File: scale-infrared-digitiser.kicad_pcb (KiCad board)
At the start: 2 copper layers, 175 x 47.5 mm, 389 parts, among them IC0 LM324PT, IC1 LM324PT, IC2 LM324PT, IC3 LM324PT, IC4 74HC4067PW,118, IC5 74HC4067PW,118, J0 Conn_02x04_TRNS, J1 Conn_02x04_RECV, Q1 T2N7002AK, Q10 T2N7002AK, Q11 T2N7002AK, Q12 T2N7002AK, Q13 T2N7002AK, Q14 T2N7002AK, Q15 T2N7002AK, Q16 T2N7002AK, Q2 T2N7002AK, Q3 T2N7002AK, Q4 T2N7002AK, Q5 T2N7002AK, Q6 T2N7002AK, Q7 T2N7002AK, Q8 T2N7002AK, Q9 T2N7002AK

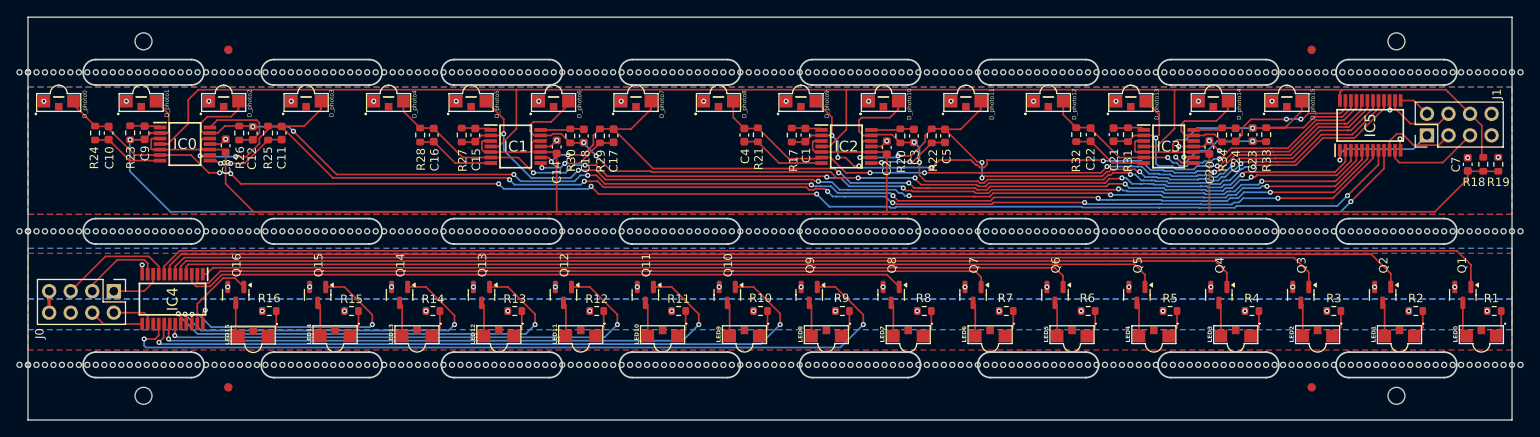
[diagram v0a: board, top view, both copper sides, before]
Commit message: revised DFM submitted to JLCPCB
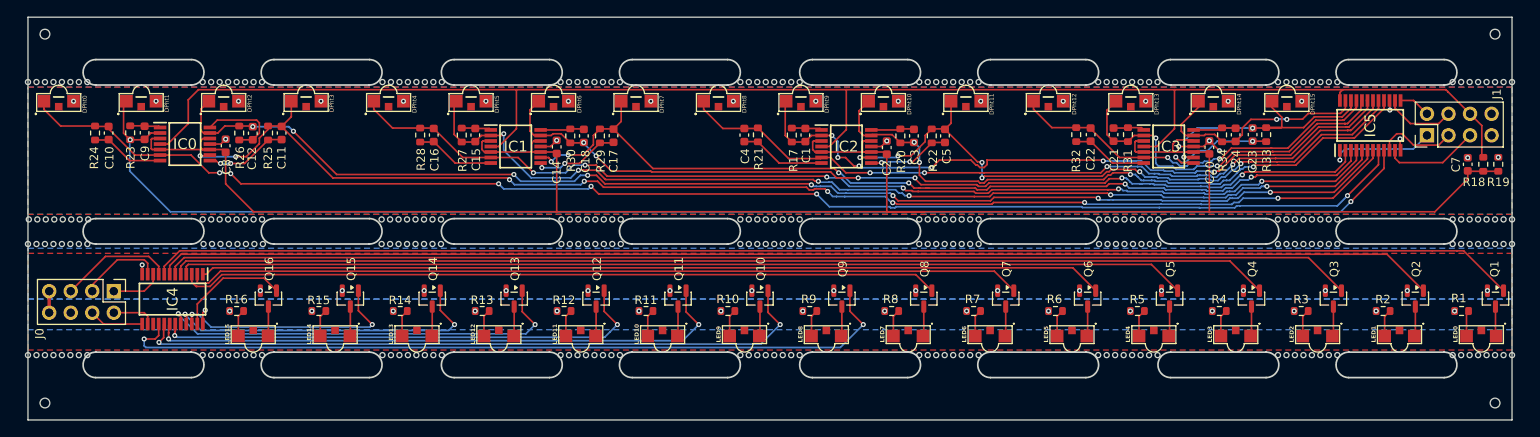
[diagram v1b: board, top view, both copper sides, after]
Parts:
- removed ? (x3): , 
- removed the REF** at (137.0, 91.2)
- removed the REF** at (173.0, 110.0)
- removed the REF** at (147.0, 110.0)
- removed the REF** at (117.0, 91.2)
- removed the REF** at (217.4, 88.6)
- removed the REF** at (103.0, 91.2)
- removed the REF** at (97.0, 125.8)
- removed the REF** at (185.0, 91.2)
- removed the REF** at (75.0, 91.2)
- removed the REF** at (131.0, 125.8)
- removed the REF** at (131.0, 110.0)
- removed the REF** at (85.0, 91.2)
- removed the REF** at (233.0, 110.0)
- removed the REF** at (123.0, 125.8)
- removed the REF** at (237.0, 91.2)
- removed the REF** at (85.0, 110.0)
- removed the REF** at (205.0, 91.2)
- removed the REF** at (201.0, 110.0)
- removed the REF** at (97.0, 110.0)
- removed the REF** at (149.0, 91.2)
- removed the REF** at (91.0, 110.0)
- removed the REF** at (185.0, 110.0)
- removed the REF** at (225.0, 110.0)
- removed the REF** at (205.0, 110.0)
- removed the REF** at (181.0, 125.8)
- removed the REF** at (121.0, 125.8)
- removed the REF** at (79.0, 125.8)
- removed the REF** at (197.0, 91.2)
- removed the REF** at (83.0, 110.0)
- removed the REF** at (183.0, 125.8)
- removed the REF** at (77.0, 110.0)
- removed the REF** at (175.0, 110.0)
- removed the REF** at (205.0, 125.8)
- removed the REF** at (71.0, 110.0)
- removed the REF** at (93.0, 91.2)
- removed the REF** at (143.0, 91.2)
- removed the REF** at (185.0, 125.8)
- removed the REF** at (127.0, 91.2)
- removed the REF** at (215.0, 110.0)
- removed the REF** at (215.0, 125.8)
- removed the REF** at (197.0, 110.0)
- removed the REF** at (89.0, 125.8)
- removed the REF** at (209.0, 125.8)
- removed the REF** at (191.0, 110.0)
- removed the REF** at (227.4, 129.4)
- removed the REF** at (219.0, 91.2)
- removed the REF** at (89.0, 91.2)
- removed the REF** at (211.0, 91.2)
- removed the REF** at (101.0, 110.0)
- removed the REF** at (183.0, 91.2)
- removed the REF** at (115.0, 125.8)
- removed the REF** at (235.0, 110.0)
- removed the REF** at (235.0, 125.8)
- removed the REF** at (119.0, 91.2)
- removed the REF** at (195.0, 125.8)
- removed the REF** at (159.0, 91.2)
- removed the REF** at (161.0, 110.0)
- removed the REF** at (123.0, 110.0)
- removed the REF** at (79.0, 91.2)
- removed the REF** at (107.0, 125.8)
- removed the REF** at (147.0, 125.8)
- removed the REF** at (227.4, 87.6)
- removed the REF** at (241.0, 110.0)
- removed the REF** at (171.0, 110.0)
- removed the REF** at (167.0, 91.2)
- removed the REF** at (223.0, 110.0)
- removed the REF** at (67.0, 125.8)
- removed the REF** at (75.0, 110.0)
- removed the REF** at (119.0, 125.8)
- removed the REF** at (211.0, 110.0)
- removed the REF** at (237.0, 110.0)
- removed the REF** at (157.0, 91.2)
- removed the REF** at (153.0, 91.2)
- removed the REF** at (197.0, 125.8)
- removed the REF** at (113.0, 125.8)
- removed the REF** at (71.0, 91.2)
- removed the REF** at (225.0, 125.8)
- removed the REF** at (227.0, 125.8)
- removed the REF** at (165.0, 110.0)
- removed the REF** at (101.0, 91.2)
- removed the REF** at (113.0, 110.0)
- removed the REF** at (91.0, 91.2)
- removed the REF** at (67.0, 91.2)
- removed the REF** at (115.0, 91.2)
- removed the REF** at (175.0, 125.8)
- removed the REF** at (105.0, 91.2)
- removed the REF** at (221.0, 125.8)
- removed the REF** at (233.0, 125.8)
- removed the REF** at (165.0, 125.8)
- removed the REF** at (111.0, 110.0)
- removed the REF** at (167.0, 125.8)
- removed the REF** at (133.0, 125.8)
- removed the REF** at (105.0, 125.8)
- removed the REF** at (169.0, 125.8)
- removed the REF** at (151.0, 91.2)
- removed the REF** at (135.0, 91.2)
- removed the REF** at (83.0, 125.8)
- removed the REF** at (151.0, 110.0)
- removed the REF** at (173.0, 125.8)
- removed the REF** at (93.0, 110.0)
- removed the REF** at (227.0, 91.2)
- removed the REF** at (71.0, 125.8)
- removed the REF** at (171.0, 91.2)
- removed the REF** at (89.6, 88.6)
- removed the REF** at (223.0, 91.2)
- removed the REF** at (89.0, 110.0)
- removed the REF** at (129.0, 125.8)
- removed the REF** at (99.0, 125.8)
- removed the REF** at (169.0, 110.0)
- removed the REF** at (111.0, 91.2)
- removed the REF** at (97.0, 91.2)
- removed the REF** at (217.0, 125.8)
- removed the REF** at (95.0, 110.0)
- removed the REF** at (229.0, 110.0)
- removed the REF** at (81.0, 110.0)
- removed the REF** at (81.0, 91.2)
- removed the REF** at (191.0, 91.2)
- removed the REF** at (109.0, 91.2)
- removed the REF** at (95.0, 91.2)
- removed the REF** at (145.0, 110.0)
- removed the REF** at (155.0, 91.2)
- removed the REF** at (111.0, 125.8)
- removed the REF** at (183.0, 110.0)
- removed the REF** at (79.6, 87.6)
- removed the REF** at (209.0, 110.0)
- removed the REF** at (201.0, 125.8)
- removed the REF** at (189.0, 110.0)
- removed the REF** at (115.0, 110.0)
- removed the REF** at (227.0, 110.0)
- removed the REF** at (229.0, 91.2)
- removed the REF** at (145.0, 91.2)
- removed the REF** at (171.0, 125.8)
- removed the REF** at (151.0, 125.8)
- removed the REF** at (211.0, 125.8)
- removed the REF** at (239.0, 91.2)
- removed the REF** at (241.0, 125.8)
- removed the REF** at (137.0, 125.8)
- removed the REF** at (155.0, 110.0)
- removed the REF** at (65.0, 91.2)
- removed the REF** at (157.0, 125.8)
- removed the REF** at (135.0, 125.8)
- removed the REF** at (207.0, 125.8)
- removed the REF** at (73.0, 110.0)
- removed the REF** at (159.0, 110.0)
- removed the REF** at (181.0, 91.2)
- removed the REF** at (135.0, 110.0)
- removed the REF** at (179.0, 125.8)
- removed the REF** at (173.0, 91.2)
- removed the REF** at (239.0, 110.0)
- removed the REF** at (121.0, 91.2)
- removed the REF** at (177.0, 91.2)
- removed the REF** at (233.0, 91.2)
- removed the REF** at (125.0, 125.8)
- removed the REF** at (161.0, 125.8)
- removed the REF** at (89.6, 128.4)
- removed the REF** at (189.0, 125.8)
- removed the REF** at (217.4, 128.4)
- removed the REF** at (137.0, 110.0)
- removed the REF** at (147.0, 91.2)
- removed the REF** at (163.0, 91.2)
- removed the REF** at (109.0, 110.0)
- removed the REF** at (163.0, 125.8)
- removed the REF** at (79.0, 110.0)
- removed the REF** at (101.0, 125.8)
- removed the REF** at (83.0, 91.2)
- removed the REF** at (181.0, 110.0)
- removed the REF** at (75.0, 125.8)
- removed the REF** at (221.0, 110.0)
- removed the REF** at (239.0, 125.8)
- removed the REF** at (179.0, 91.2)
- removed the REF** at (133.0, 110.0)
- removed the REF** at (65.0, 110.0)
- removed the REF** at (207.0, 110.0)
- removed the REF** at (189.0, 91.2)
- removed the REF** at (209.0, 91.2)
- removed the REF** at (237.0, 125.8)
- removed the REF** at (131.0, 91.2)
- removed the REF** at (117.0, 110.0)
- removed the REF** at (177.0, 110.0)
- removed the REF** at (175.0, 91.2)
- removed the REF** at (77.0, 125.8)
- removed the REF** at (123.0, 91.2)
- removed the REF** at (215.0, 91.2)
- removed the REF** at (103.0, 110.0)
- removed the REF** at (73.0, 91.2)
- removed the REF** at (95.0, 125.8)
- removed the REF** at (203.0, 125.8)
- removed the REF** at (77.0, 91.2)
- removed the REF** at (67.0, 110.0)
- removed the REF** at (155.0, 125.8)
- removed the REF** at (187.0, 91.2)
- removed the REF** at (163.0, 110.0)
- removed the REF** at (143.0, 110.0)
- removed the REF** at (87.0, 91.2)
- removed the REF** at (219.0, 110.0)
- removed the REF** at (191.0, 125.8)
- removed the REF** at (221.0, 91.2)
- removed the REF** at (133.0, 91.2)
- removed the REF** at (103.0, 125.8)
- removed the REF** at (65.0, 125.8)
- removed the REF** at (199.0, 110.0)
- removed the REF** at (141.0, 91.2)
- removed the REF** at (139.0, 110.0)
- removed the REF** at (153.0, 125.8)
- removed the REF** at (125.0, 110.0)
- removed the REF** at (69.0, 110.0)
- removed the REF** at (223.0, 125.8)
- removed the REF** at (145.0, 125.8)
- removed the REF** at (125.0, 91.2)
- removed the REF** at (195.0, 91.2)
- removed the REF** at (213.0, 91.2)
- removed the REF** at (99.0, 110.0)
- removed the REF** at (203.0, 110.0)
- removed the REF** at (69.0, 91.2)
- removed the REF** at (79.6, 129.4)
- removed the REF** at (127.0, 110.0)
- removed the REF** at (217.0, 110.0)
- removed the REF** at (187.0, 125.8)
- removed the REF** at (203.0, 91.2)
- removed the REF** at (235.0, 91.2)
- removed the REF** at (87.0, 125.8)
- removed the REF** at (129.0, 110.0)
- removed the REF** at (207.0, 91.2)
- removed the REF** at (217.0, 91.2)
- removed the REF** at (91.0, 125.8)
- removed the REF** at (193.0, 91.2)
- removed the REF** at (85.0, 125.8)
- removed the REF** at (117.0, 125.8)
- removed the REF** at (179.0, 110.0)
- removed the REF** at (231.0, 91.2)
- removed the REF** at (199.0, 125.8)
- removed the REF** at (139.0, 125.8)
- removed the REF** at (241.0, 91.2)
- removed the REF** at (231.0, 110.0)
- removed the REF** at (69.0, 125.8)
- removed the REF** at (159.0, 125.8)
- removed the REF** at (199.0, 91.2)
- removed the REF** at (107.0, 91.2)
- removed the REF** at (187.0, 110.0)
- removed the REF** at (149.0, 125.8)
- removed the REF** at (99.0, 91.2)
- removed the REF** at (143.0, 125.8)
- removed the REF** at (73.0, 125.8)
- removed the REF** at (141.0, 125.8)
- removed the REF** at (201.0, 91.2)
- removed the REF** at (193.0, 125.8)
- removed the REF** at (177.0, 125.8)
- removed the REF** at (195.0, 110.0)
- removed the REF** at (149.0, 110.0)
- removed the REF** at (157.0, 110.0)
- removed the REF** at (167.0, 110.0)
- removed the REF** at (129.0, 91.2)
- removed the REF** at (107.0, 110.0)
- removed the REF** at (109.0, 125.8)
- removed the REF** at (113.0, 91.2)
- removed the REF** at (141.0, 110.0)
- removed the REF** at (225.0, 91.2)
- removed the REF** at (121.0, 110.0)
- removed the REF** at (169.0, 91.2)
- removed the REF** at (213.0, 110.0)
- removed the REF** at (213.0, 125.8)
- removed the REF** at (93.0, 125.8)
- removed the REF** at (153.0, 110.0)
- removed the REF** at (139.0, 91.2)
- removed the REF** at (87.0, 110.0)
- removed the REF** at (127.0, 125.8)
- removed the REF** at (229.0, 125.8)
- removed the REF** at (219.0, 125.8)
- removed the REF** at (193.0, 110.0)
- removed the REF** at (81.0, 125.8)
- removed the REF** at (105.0, 110.0)
- removed the REF** at (231.0, 125.8)
- removed the REF** at (161.0, 91.2)
- removed the REF** at (165.0, 91.2)
- removed the REF** at (119.0, 110.0)
- added REF**: mouse_bites, manufacturing:mouse_bites, F.Cu at (234.0, 92.4)
- added REF**: mouse_bites, manufacturing:mouse_bites, F.Cu at (128.8, 92.4)
- added REF**: mouse_bites, manufacturing:mouse_bites, F.Cu at (92.6, 92.4)
- added REF**: mouse_bites, manufacturing:mouse_bites, F.Cu at (213.4, 92.4)
- added REF**: mouse_bites, manufacturing:mouse_bites, F.Cu at (133.8, 124.6)
- added REF**: mouse_bites, manufacturing:mouse_bites, F.Cu at (177.1, 108.6)
- added REF**: mouse_bites, manufacturing:mouse_bites, F.Cu at (128.8, 124.6)
- added REF**: mouse_bites, manufacturing:mouse_bites, F.Cu at (134.9, 108.6)
- added REF**: mouse_bites, manufacturing:mouse_bites, F.Cu at (156.0, 92.4)
- added REF**: mouse_bites, manufacturing:mouse_bites, F.Cu at (113.7, 108.6)
- added REF**: mouse_bites, manufacturing:mouse_bites, F.Cu at (199.2, 124.6)
- added REF**: mouse_bites, manufacturing:mouse_bites, F.Cu at (66.0, 111.5)
- added REF**: mouse_bites, manufacturing:mouse_bites, F.Cu at (112.7, 108.6)
- added REF**: mouse_bites, manufacturing:mouse_bites, F.Cu at (171.1, 124.6)
- added REF**: mouse_bites, manufacturing:mouse_bites, F.Cu at (239.0, 111.5)
- added REF**: mouse_bites, manufacturing:mouse_bites, F.Cu at (237.0, 124.6)
- added REF**: mouse_bites, manufacturing:mouse_bites, F.Cu at (218.4, 111.5)
- added REF**: mouse_bites, manufacturing:mouse_bites, F.Cu at (134.9, 111.5)
- added REF**: ToolingHole_1.152mm, MountingHole:ToolingHole_1.152mm, F.Cu at (68.0, 86.8)
- added REF**: mouse_bites, manufacturing:mouse_bites, F.Cu at (91.7, 111.5)
- added REF**: mouse_bites, manufacturing:mouse_bites, F.Cu at (219.4, 124.6)
- added REF**: mouse_bites, manufacturing:mouse_bites, F.Cu at (112.8, 124.6)
- added REF**: mouse_bites, manufacturing:mouse_bites, F.Cu at (69.0, 111.5)
- added REF**: mouse_bites, manufacturing:mouse_bites, F.Cu at (234.0, 108.6)
- added REF**: mouse_bites, manufacturing:mouse_bites, F.Cu at (112.7, 111.5)
- added REF**: mouse_bites, manufacturing:mouse_bites, F.Cu at (176.1, 92.4)
- added REF**: mouse_bites, manufacturing:mouse_bites, F.Cu at (69.0, 124.6)
- added REF**: mouse_bites, manufacturing:mouse_bites, F.Cu at (237.0, 111.5)
- added REF**: mouse_bites, manufacturing:mouse_bites, F.Cu at (213.4, 111.5)
- added REF**: mouse_bites, manufacturing:mouse_bites, F.Cu at (113.8, 124.6)
- added REF**: mouse_bites, manufacturing:mouse_bites, F.Cu at (150.0, 92.4)
- added REF**: mouse_bites, manufacturing:mouse_bites, F.Cu at (194.2, 124.6)
- added REF**: mouse_bites, manufacturing:mouse_bites, F.Cu at (171.1, 111.5)
- added REF**: mouse_bites, manufacturing:mouse_bites, F.Cu at (197.3, 108.6)
- added REF**: mouse_bites, manufacturing:mouse_bites, F.Cu at (197.3, 111.5)
- added REF**: mouse_bites, manufacturing:mouse_bites, F.Cu at (216.4, 92.4)
- added REF**: mouse_bites, manufacturing:mouse_bites, F.Cu at (107.7, 111.5)
- added REF**: mouse_bites, manufacturing:mouse_bites, F.Cu at (240.0, 124.6)
- added REF**: mouse_bites, manufacturing:mouse_bites, F.Cu at (234.0, 111.5)
- added REF**: mouse_bites, manufacturing:mouse_bites, F.Cu at (174.1, 92.4)
- added REF**: mouse_bites, manufacturing:mouse_bites, F.Cu at (69.1, 108.6)
- added REF**: mouse_bites, manufacturing:mouse_bites, F.Cu at (155.0, 92.4)
- added REF**: mouse_bites, manufacturing:mouse_bites, F.Cu at (72.0, 124.6)
- added REF**: mouse_bites, manufacturing:mouse_bites, F.Cu at (71.0, 92.4)
- added REF**: mouse_bites, manufacturing:mouse_bites, F.Cu at (237.0, 108.6)
- added REF**: mouse_bites, manufacturing:mouse_bites, F.Cu at (213.4, 124.6)
- added REF**: mouse_bites, manufacturing:mouse_bites, F.Cu at (69.0, 92.4)
- added REF**: mouse_bites, manufacturing:mouse_bites, F.Cu at (239.0, 108.6)
- added REF**: mouse_bites, manufacturing:mouse_bites, F.Cu at (110.7, 111.5)
- added REF**: mouse_bites, manufacturing:mouse_bites, F.Cu at (107.8, 92.4)
- added REF**: mouse_bites, manufacturing:mouse_bites, F.Cu at (89.7, 111.5)
- added REF**: mouse_bites, manufacturing:mouse_bites, F.Cu at (153.0, 124.6)
- added REF**: mouse_bites, manufacturing:mouse_bites, F.Cu at (156.0, 108.6)
- added REF**: mouse_bites, manufacturing:mouse_bites, F.Cu at (194.2, 92.4)
- added REF**: mouse_bites, manufacturing:mouse_bites, F.Cu at (92.6, 124.6)
- added REF**: mouse_bites, manufacturing:mouse_bites, F.Cu at (177.1, 111.5)
- added REF**: mouse_bites, manufacturing:mouse_bites, F.Cu at (219.4, 111.5)
- added REF**: mouse_bites, manufacturing:mouse_bites, F.Cu at (131.9, 111.5)
- added REF**: mouse_bites, manufacturing:mouse_bites, F.Cu at (133.9, 111.5)
- added REF**: mouse_bites, manufacturing:mouse_bites, F.Cu at (72.0, 111.5)
- added REF**: mouse_bites, manufacturing:mouse_bites, F.Cu at (171.1, 92.4)
- added REF**: mouse_bites, manufacturing:mouse_bites, F.Cu at (153.0, 92.4)
- added REF**: mouse_bites, manufacturing:mouse_bites, F.Cu at (134.8, 124.6)
- added REF**: mouse_bites, manufacturing:mouse_bites, F.Cu at (71.0, 111.5)
- added REF**: mouse_bites, manufacturing:mouse_bites, F.Cu at (150.0, 124.6)
- added REF**: mouse_bites, manufacturing:mouse_bites, F.Cu at (239.0, 124.6)
- added REF**: mouse_bites, manufacturing:mouse_bites, F.Cu at (91.6, 124.6)
- added REF**: mouse_bites, manufacturing:mouse_bites, F.Cu at (174.1, 111.5)
- added REF**: mouse_bites, manufacturing:mouse_bites, F.Cu at (72.1, 108.6)
- added REF**: mouse_bites, manufacturing:mouse_bites, F.Cu at (195.3, 108.6)
- added REF**: mouse_bites, manufacturing:mouse_bites, F.Cu at (86.6, 108.6)
- added REF**: mouse_bites, manufacturing:mouse_bites, F.Cu at (150.0, 111.5)
- added REF**: mouse_bites, manufacturing:mouse_bites, F.Cu at (155.0, 111.5)
- added REF**: mouse_bites, manufacturing:mouse_bites, F.Cu at (216.4, 124.6)
- added REF**: mouse_bites, manufacturing:mouse_bites, F.Cu at (89.6, 124.6)
- added REF**: mouse_bites, manufacturing:mouse_bites, F.Cu at (216.4, 108.6)
- added REF**: mouse_bites, manufacturing:mouse_bites, F.Cu at (240.0, 92.4)
- added REF**: mouse_bites, manufacturing:mouse_bites, F.Cu at (86.7, 111.5)
- added REF**: mouse_bites, manufacturing:mouse_bites, F.Cu at (155.0, 108.6)
- added REF**: mouse_bites, manufacturing:mouse_bites, F.Cu at (219.4, 108.6)
- added REF**: mouse_bites, manufacturing:mouse_bites, F.Cu at (174.1, 108.6)
- added REF**: mouse_bites, manufacturing:mouse_bites, F.Cu at (240.0, 111.5)
- added REF**: mouse_bites, manufacturing:mouse_bites, F.Cu at (192.3, 111.5)
- added REF**: mouse_bites, manufacturing:mouse_bites, F.Cu at (177.1, 92.4)
- added REF**: mouse_bites, manufacturing:mouse_bites, F.Cu at (113.8, 92.4)
- added REF**: mouse_bites, manufacturing:mouse_bites, F.Cu at (174.1, 124.6)
- added REF**: mouse_bites, manufacturing:mouse_bites, F.Cu at (150.0, 108.6)
- added REF**: mouse_bites, manufacturing:mouse_bites, F.Cu at (91.6, 92.4)
- added REF**: mouse_bites, manufacturing:mouse_bites, F.Cu at (192.3, 108.6)
- added REF**: mouse_bites, manufacturing:mouse_bites, F.Cu at (131.8, 124.6)
- added REF**: mouse_bites, manufacturing:mouse_bites, F.Cu at (134.8, 92.4)
- added REF**: mouse_bites, manufacturing:mouse_bites, F.Cu at (89.6, 108.6)
- added REF**: mouse_bites, manufacturing:mouse_bites, F.Cu at (198.3, 111.5)
- added REF**: mouse_bites, manufacturing:mouse_bites, F.Cu at (153.0, 108.6)
- added REF**: mouse_bites, manufacturing:mouse_bites, F.Cu at (110.7, 108.6)
- added REF**: mouse_bites, manufacturing:mouse_bites, F.Cu at (176.1, 108.6)
- added REF**: mouse_bites, manufacturing:mouse_bites, F.Cu at (110.8, 92.4)
- added REF**: mouse_bites, manufacturing:mouse_bites, F.Cu at (156.0, 124.6)
- added REF**: mouse_bites, manufacturing:mouse_bites, F.Cu at (193.2, 124.6)
- added REF**: mouse_bites, manufacturing:mouse_bites, F.Cu at (128.9, 108.6)
- added REF**: mouse_bites, manufacturing:mouse_bites, F.Cu at (133.8, 92.4)
- added REF**: mouse_bites, manufacturing:mouse_bites, F.Cu at (71.1, 108.6)
- added REF**: mouse_bites, manufacturing:mouse_bites, F.Cu at (107.7, 108.6)
- added REF**: mouse_bites, manufacturing:mouse_bites, F.Cu at (89.6, 92.4)
- added REF**: mouse_bites, manufacturing:mouse_bites, F.Cu at (218.4, 124.6)
- added REF**: mouse_bites, manufacturing:mouse_bites, F.Cu at (66.1, 108.6)
- added REF**: mouse_bites, manufacturing:mouse_bites, F.Cu at (131.9, 108.6)
- added REF**: mouse_bites, manufacturing:mouse_bites, F.Cu at (71.0, 124.6)
- added REF**: mouse_bites, manufacturing:mouse_bites, F.Cu at (176.1, 111.5)
- added REF**: mouse_bites, manufacturing:mouse_bites, F.Cu at (237.0, 92.4)
- added REF**: mouse_bites, manufacturing:mouse_bites, F.Cu at (66.0, 124.6)
- added REF**: mouse_bites, manufacturing:mouse_bites, F.Cu at (107.8, 124.6)
- added REF**: mouse_bites, manufacturing:mouse_bites, F.Cu at (156.0, 111.5)
- added REF**: mouse_bites, manufacturing:mouse_bites, F.Cu at (112.8, 92.4)
- added REF**: ToolingHole_1.152mm, MountingHole:ToolingHole_1.152mm, F.Cu at (239.0, 86.8)
- added REF**: mouse_bites, manufacturing:mouse_bites, F.Cu at (171.1, 108.6)
- added REF**: mouse_bites, manufacturing:mouse_bites, F.Cu at (196.2, 92.4)
- added REF**: mouse_bites, manufacturing:mouse_bites, F.Cu at (213.4, 108.6)
- added REF**: mouse_bites, manufacturing:mouse_bites, F.Cu at (216.4, 111.5)
- added REF**: mouse_bites, manufacturing:mouse_bites, F.Cu at (176.1, 124.6)
- added REF**: mouse_bites, manufacturing:mouse_bites, F.Cu at (133.9, 108.6)
- added REF**: mouse_bites, manufacturing:mouse_bites, F.Cu at (66.0, 92.4)
- added REF**: mouse_bites, manufacturing:mouse_bites, F.Cu at (198.3, 108.6)
- added REF**: mouse_bites, manufacturing:mouse_bites, F.Cu at (240.0, 108.6)
- added REF**: mouse_bites, manufacturing:mouse_bites, F.Cu at (199.2, 92.4)
- added REF**: mouse_bites, manufacturing:mouse_bites, F.Cu at (113.7, 111.5)
- added REF**: mouse_bites, manufacturing:mouse_bites, F.Cu at (193.2, 92.4)
- added REF**: mouse_bites, manufacturing:mouse_bites, F.Cu at (155.0, 124.6)
- added REF**: mouse_bites, manufacturing:mouse_bites, F.Cu at (86.6, 92.4)
- added REF**: mouse_bites, manufacturing:mouse_bites, F.Cu at (234.0, 124.6)
- added REF**: mouse_bites, manufacturing:mouse_bites, F.Cu at (218.4, 92.4)
- added REF**: mouse_bites, manufacturing:mouse_bites, F.Cu at (239.0, 92.4)
- added REF**: mouse_bites, manufacturing:mouse_bites, F.Cu at (86.6, 124.6)
- added REF**: mouse_bites, manufacturing:mouse_bites, F.Cu at (131.8, 92.4)
- added REF**: mouse_bites, manufacturing:mouse_bites, F.Cu at (177.1, 124.6)
- added REF**: mouse_bites, manufacturing:mouse_bites, F.Cu at (195.3, 111.5)
- added REF**: ToolingHole_1.152mm, MountingHole:ToolingHole_1.152mm, F.Cu at (239.0, 130.2)
- added REF**: mouse_bites, manufacturing:mouse_bites, F.Cu at (153.0, 111.5)
- added REF**: mouse_bites, manufacturing:mouse_bites, F.Cu at (110.8, 124.6)
- added REF**: mouse_bites, manufacturing:mouse_bites, F.Cu at (72.0, 92.4)
- added REF**: mouse_bites, manufacturing:mouse_bites, F.Cu at (92.6, 108.6)
- added REF**: mouse_bites, manufacturing:mouse_bites, F.Cu at (128.9, 111.5)
- added REF**: mouse_bites, manufacturing:mouse_bites, F.Cu at (218.4, 108.6)
- added REF**: ToolingHole_1.152mm, MountingHole:ToolingHole_1.152mm, F.Cu at (68.0, 130.2)
- added REF**: mouse_bites, manufacturing:mouse_bites, F.Cu at (92.7, 111.5)
- added REF**: mouse_bites, manufacturing:mouse_bites, F.Cu at (219.4, 92.4)
- added REF**: mouse_bites, manufacturing:mouse_bites, F.Cu at (196.2, 124.6)
- added REF**: mouse_bites, manufacturing:mouse_bites, F.Cu at (91.6, 108.6)
- moved Q1 3.87 mm to (239.1, 117.9)
- moved Q10 3.87 mm to (152.3, 117.9)
- moved Q3 3.87 mm to (219.9, 117.9)
- moved Q13 3.87 mm to (123.3, 117.9)
- moved Q14 3.87 mm to (113.7, 117.9)
- moved Q11 3.87 mm to (142.7, 117.9)
- moved Q12 3.87 mm to (133.0, 117.9)
- moved Q15 3.87 mm to (104.0, 117.9)
- moved Q16 3.87 mm to (94.3, 117.9)
- moved Q2 3.87 mm to (229.6, 117.9)
- moved Q4 3.87 mm to (210.3, 117.9)
- moved Q5 3.87 mm to (200.6, 117.9)
- moved Q6 3.87 mm to (191.0, 117.9)
- moved Q7 3.87 mm to (181.3, 117.9)
- moved Q8 3.87 mm to (171.6, 117.9)
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- renumbered D_photo0 to DPht0, D_photo1 to DPht1, D_photo10 to DPht10, D_photo11 to DPht11, D_photo12 to DPht12, D_photo13 to DPht13, D_photo14 to DPht14, D_photo15 to DPht15, D_photo2 to DPht2, D_photo3 to DPht3, D_photo4 to DPht4, D_photo5 to DPht5, D_photo6 to DPht6, D_photo7 to DPht7, D_photo8 to DPht8, D_photo9 to DPht9
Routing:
- net /LED_CTL_7: track 85.7 -> 89.8 mm
- net /LED_CTL_15: track 9.55 -> 13.6 mm
- net /PHT_DAT_1: track 163.6 -> 167.5 mm
- net /PHT_DAT_15: track 79.5 -> 76.1 mm
- net /PHT_DAT_5: track 121.6 -> 125.0 mm
- net /LED_CTL_6: track 95.4 -> 98.8 mm
- net /LED_CTL_14: track 31.2 -> 27.9 mm
- net /LED_CTL_13: track 42.1 -> 38.8 mm
- net /LED_CTL_12: track 52.8 -> 49.5 mm
- net /LED_CTL_11: track 62.2 -> 58.9 mm
- net /LED_CTL_10: track 73.1 -> 69.8 mm
- net /LED_CTL_9: track 84.6 -> 81.3 mm
- net /LED_CTL_8: track 98.0 -> 94.7 mm
- net /LED_CTL_5: track 103.5 -> 106.7 mm
- net /LED_CTL_4: track 116.0 -> 119.2 mm
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
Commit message: modifying prototype
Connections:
- net Net-(IC0-OUTPUT_1) renamed /PHT_DAT_0_R
- net Net-(IC0-OUTPUT_2) renamed /PHT_DAT_1_R
- net Net-(IC0-OUTPUT_3) renamed /PHT_DAT_2_R
- net Net-(IC0-OUTPUT_4) renamed /PHT_DAT_3_R
- net Net-(IC1-OUTPUT_1) renamed /PHT_DAT_4_R
- net Net-(IC1-OUTPUT_2) renamed /PHT_DAT_5_R
- net Net-(IC1-OUTPUT_3) renamed /PHT_DAT_6_R
- net Net-(IC1-OUTPUT_4) renamed /PHT_DAT_7_R
- net Net-(IC2-OUTPUT_1) renamed /PHT_DAT_12_R
- net Net-(IC2-OUTPUT_2) renamed /PHT_DAT_13_R
- net Net-(IC2-OUTPUT_3) renamed /PHT_DAT_14_R
- net Net-(IC2-OUTPUT_4) renamed /PHT_DAT_15_R
- net Net-(IC3-OUTPUT_1) renamed /PHT_DAT_11_R
- net Net-(IC3-OUTPUT_2) renamed /PHT_DAT_10_R
- net Net-(IC3-OUTPUT_3) renamed /PHT_DAT_9_R
- net Net-(IC3-OUTPUT_4) renamed /PHT_DAT_8_R
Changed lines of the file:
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@@
 	)
 	(net 0 "")
-	(net 1 "Net-(IC2-OUTPUT_1)")
+	(net 1 "/PHT_DAT_12_R")
 	(net 2 "/PHT_DAT_12")
 	(net 3 "/NON_INVERTING_REF")
 	(net 4 "GND")
-	(net 5 "Net-(IC2-OUTPUT_4)")
+	(net 5 "/PHT_DAT_15_R")
 	(net 6 "/PHT_DAT_15")
 	(net 7 "/PHT_DAT_13")
-	(net 8 "Net-(IC2-OUTPUT_2)")
+	(net 8 "/PHT_DAT_13_R")
 	(net 9 "/PHT_DAT_14")
-	(net 10 "Net-(IC2-OUTPUT_3)")
+	(net 10 "/PHT_DAT_14_R")
 	(net 11 "/PHT_DAT_0")
-	(net 12 "Net-(IC0-OUTPUT_1)")
+	(net 12 "/PHT_DAT_0_R")
 	(net 13 "/PHT_DAT_1")
-	(net 14 "Net-(IC0-OUTPUT_2)")
-	(net 15 "Net-(IC0-OUTPUT_3)")
+	(net 14 "/PHT_DAT_1_R")
+	(net 15 "/PHT_DAT_2_R")
 	(net 16 "/PHT_DAT_2")
 	(net 17 "/PHT_DAT_3")
-	(net 18 "Net-(IC0-OUTPUT_4)")
-	(net 19 "Net-(IC1-OUTPUT_1)")
+	(net 18 "/PHT_DAT_3_R")
+	(net 19 "/PHT_DAT_4_R")
 	(net 20 "/PHT_DAT_4")
 	(net 21 "/PHT_DAT_5")
-	(net 22 "Net-(IC1-OUTPUT_2)")
+	(net 22 "/PHT_DAT_5_R")
 	(net 23 "/PHT_DAT_6")
-	(net 24 "Net-(IC1-OUTPUT_3)")
+	(net 24 "/PHT_DAT_6_R")
 	(net 25 "/PHT_DAT_7")
-	(net 26 "Net-(IC1-OUTPUT_4)")
+	(net 26 "/PHT_DAT_7_R")
 	(net 27 "/PHT_DAT_8")
-	(net 28 "Net-(IC3-OUTPUT_1)")
+	(net 28 "/PHT_DAT_11_R")
 	(net 29 "/PHT_DAT_9")
-	(net 30 "Net-(IC3-OUTPUT_2)")
+	(net 30 "/PHT_DAT_10_R")
 	(net 31 "/PHT_DAT_10")
-	(net 32 "Net-(IC3-OUTPUT_3)")
-	(net 33 "Net-(IC3-OUTPUT_4)")
+	(net 32 "/PHT_DAT_9_R")
+	(net 33 "/PHT_DAT_8_R")
 	(net 34 "/PHT_DAT_11")
 	(net 35 "unconnected-(DPht0-EP-Pad3)")
@@
 			(layers "F.Cu" "F.Mask" "F.Paste")
 			(roundrect_rratio 0.25)
-			(net 18 "Net-(IC0-OUTPUT_4)")
+			(net 18 "/PHT_DAT_3_R")
 			(pintype "passive")
 		)
@@
 			(layers "F.Cu" "F.Mask" "F.Paste")
 			(roundrect_rratio 0.25)
-			(net 1 "Net-(IC2-OUTPUT_1)")
+			(net 1 "/PHT_DAT_12_R")
 			(pintype "passive")
 		)
@@
 			(layers "F.Cu" "F.Mask" "F.Paste")
 			(roundrect_rratio 0.25)
-			(net 33 "Net-(IC3-OUTPUT_4)")
+			(net 33 "/PHT_DAT_8_R")
 			(pintype "passive")
 		)
@@
 			(size 0.45 1.475)
 			(layers "F.Cu" "F.Mask" "F.Paste")
-			(net 28 "Net-(IC3-OUTPUT_1)")
+			(net 28 "/PHT_DAT_11_R")
 			(pinfunction "OUTPUT_1")
 			(pintype "passive")
@@
 			(size 0.45 1.475)
 			(layers "F.Cu" "F.Mask" "F.Paste")
-			(net 30 "Net-(IC3-OUTPUT_2)")
+			(net 30 "/PHT_DAT_10_R")
 			(pinfunction "OUTPUT_2")
 			(pintype "passive")
@@
 			(size 0.45 1.475)
 			(layers "F.Cu" "F.Mask" "F.Paste")
-			(net 32 "Net-(IC3-OUTPUT_3)")
+			(net 32 "/PHT_DAT_9_R")
 			(pinfunction "OUTPUT_3")
 			(pintype "passive")
@@
 			(size 0.45 1.475)
 			(layers "F.Cu" "F.Mask" "F.Paste")
-			(net 33 "Net-(IC3-OUTPUT_4)")
+			(net 33 "/PHT_DAT_8_R")
 			(pinfunction "OUTPUT_4")
 			(pintype "passive")
@@
 			(layers "F.Cu" "F.Mask" "F.Paste")
 			(roundrect_rratio 0.25)
-			(net 10 "Net-(IC2-OUTPUT_3)")
+			(net 10 "/PHT_DAT_14_R")
 			(pintype "passive")
 		)
@@
 			(size 0.45 1.475)
 			(layers "F.Cu" "F.Mask" "F.Paste")
-			(net 12 "Net-(IC0-OUTPUT_1)")
+			(net 12 "/PHT_DAT_0_R")
 			(pinfunction "OUTPUT_1")
 			(pintype "passive")
@@
 			(size 0.45 1.475)
 			(layers "F.Cu" "F.Mask" "F.Paste")
-			(net 14 "Net-(IC0-OUTPUT_2)")
+			(net 14 "/PHT_DAT_1_R")
 			(pinfunction "OUTPUT_2")
 			(pintype "passive")
@@
 			(size 0.45 1.475)
 			(layers "F.Cu" "F.Mask" "F.Paste")
-			(net 15 "Net-(IC0-OUTPUT_3)")
+			(net 15 "/PHT_DAT_2_R")
 			(pinfunction "OUTPUT_3")
 			(pintype "passive")
@@
 			(size 0.45 1.475)
 			(layers "F.Cu" "F.Mask" "F.Paste")
-			(net 18 "Net-(IC0-OUTPUT_4)")
+			(net 18 "/PHT_DAT_3_R")
 			(pinfunction "OUTPUT_4")
 			(pintype "passive")
@@
 			(layers "F.Cu" "F.Mask" "F.Paste")
 			(roundrect_rratio 0.25)
-			(net 15 "Net-(IC0-OUTPUT_3)")
+			(net 15 "/PHT_DAT_2_R")
 			(pintype "passive")
 		)
@@
 			(size 0.45 1.475)
 			(layers "F.Cu" "F.Mask" "F.Paste")
-			(net 1 "Net-(IC2-OUTPUT_1)")
+			(net 1 "/PHT_DAT_12_R")
 			(pinfunction "OUTPUT_1")
 			(pintype "passive")
@@
 			(size 0.45 1.475)
 			(layers "F.Cu" "F.Mask" "F.Paste")
-			(net 8 "Net-(IC2-OUTPUT_2)")
+			(net 8 "/PHT_DAT_13_R")
 			(pinfunction "OUTPUT_2")
 			(pintype "passive")
@@
 			(size 0.45 1.475)
 			(layers "F.Cu" "F.Mask" "F.Paste")
-			(net 10 "Net-(IC2-OUTPUT_3)")
+			(net 10 "/PHT_DAT_14_R")
 			(pinfunction "OUTPUT_3")
 			(pintype "passive")
@@
 			(size 0.45 1.475)
 			(layers "F.Cu" "F.Mask" "F.Paste")
-			(net 5 "Net-(IC2-OUTPUT_4)")
+			(net 5 "/PHT_DAT_15_R")
 			(pinfunction "OUTPUT_4")
 			(pintype "passive")
@@
 			(size 0.45 1.475)
 			(layers "F.Cu" "F.Mask" "F.Paste")
-			(net 19 "Net-(IC1-OUTPUT_1)")
+			(net 19 "/PHT_DAT_4_R")
 			(pinfunction "OUTPUT_1")
 			(pintype "passive")
@@
 			(size 0.45 1.475)
 			(layers "F.Cu" "F.Mask" "F.Paste")
-			(net 22 "Net-(IC1-OUTPUT_2)")
+			(net 22 "/PHT_DAT_5_R")
 			(pinfunction "OUTPUT_2")
 			(pintype "passive")
@@
 			(size 0.45 1.475)
 			(layers "F.Cu" "F.Mask" "F.Paste")
-			(net 24 "Net-(IC1-OUTPUT_3)")
+			(net 24 "/PHT_DAT_6_R")
 			(pinfunction "OUTPUT_3")
 			(pintype "passive")
@@
 			(size 0.45 1.475)
 			(layers "F.Cu" "F.Mask" "F.Paste")
-			(net 26 "Net-(IC1-OUTPUT_4)")
+			(net 26 "/PHT_DAT_7_R")
 			(pinfunction "OUTPUT_4")
 			(pintype "passive")
@@
 			(layers "F.Cu" "F.Mask" "F.Paste")
 			(roundrect_rratio 0.25)
-			(net 19 "Net-(IC1-OUTPUT_1)")
+			(net 19 "/PHT_DAT_4_R")
 			(pintype "passive")
 		)
@@
 			(layers "F.Cu" "F.Mask" "F.Paste")
 			(roundrect_rratio 0.25)
-			(net 24 "Net-(IC1-OUTPUT_3)")
+			(net 24 "/PHT_DAT_6_R")
 			(pintype "passive")
 		)
@@
 			(layers "F.Cu" "F.Mask" "F.Paste")
 			(roundrect_rratio 0.25)
-			(net 12 "Net-(IC0-OUTPUT_1)")
+			(net 12 "/PHT_DAT_0_R")
 			(pintype "passive")
 		)
@@
 			(layers "F.Cu" "F.Mask" "F.Paste")
 			(roundrect_rratio 0.25)
-			(net 33 "Net-(IC3-OUTPUT_4)")
+			(net 33 "/PHT_DAT_8_R")
 			(pintype "passive")
 		)
@@
 			(layers "F.Cu" "F.Mask" "F.Paste")
 			(roundrect_rratio 0.25)
-			(net 15 "Net-(IC0-OUTPUT_3)")
+			(net 15 "/PHT_DAT_2_R")
 			(pintype "passive")
 		)
@@
 			(layers "F.Cu" "F.Mask" "F.Paste")
 			(roundrect_rratio 0.25)
-			(net 19 "Net-(IC1-OUTPUT_1)")
+			(net 19 "/PHT_DAT_4_R")
 			(pintype "passive")
 		)
@@
 			(layers "F.Cu" "F.Mask" "F.Paste")
 			(roundrect_rratio 0.25)
-			(net 28 "Net-(IC3-OUTPUT_1)")
+			(net 28 "/PHT_DAT_11_R")
 			(pintype "passive")
 		)
@@
 			(layers "F.Cu" "F.Mask" "F.Paste")
 			(roundrect_rratio 0.25)
-			(net 32 "Net-(IC3-OUTPUT_3)")
+			(net 32 "/PHT_DAT_9_R")
 			(pintype "passive")
 		)
@@
 			(layers "F.Cu" "F.Mask" "F.Paste")
 			(roundrect_rratio 0.25)
-			(net 32 "Net-(IC3-OUTPUT_3)")
+			(net 32 "/PHT_DAT_9_R")
 			(pintype "passive")
 		)
@@
 			(layers "F.Cu" "F.Mask" "F.Paste")
 			(roundrect_rratio 0.25)
-			(net 14 "Net-(IC0-OUTPUT_2)")
+			(net 14 "/PHT_DAT_1_R")
 			(pintype "passive")
 		)
@@
 			(layers "F.Cu" "F.Mask" "F.Paste")
 			(roundrect_rratio 0.25)
-			(net 8 "Net-(IC2-OUTPUT_2)")
+			(net 8 "/PHT_DAT_13_R")
 			(pintype "passive")
 		)
@@
 			(layers "F.Cu" "F.Mask" "F.Paste")
 			(roundrect_rratio 0.25)
-			(net 30 "Net-(IC3-OUTPUT_2)")
+			(net 30 "/PHT_DAT_10_R")
 			(pintype "passive")
 		)
@@
 			(layers "F.Cu" "F.Mask" "F.Paste")
 			(roundrect_rratio 0.25)
-			(net 24 "Net-(IC1-OUTPUT_3)")
+			(net 24 "/PHT_DAT_6_R")
 			(pintype "passive")
 		)
@@
 			(layers "F.Cu" "F.Mask" "F.Paste")
 			(roundrect_rratio 0.25)
-			(net 30 "Net-(IC3-OUTPUT_2)")
+			(net 30 "/PHT_DAT_10_R")
 			(pintype "passive")
 		)
@@
 			(layers "F.Cu" "F.Mask" "F.Paste")
 			(roundrect_rratio 0.25)
-			(net 12 "Net-(IC0-OUTPUT_1)")
+			(net 12 "/PHT_DAT_0_R")
 			(pintype "passive")
 		)
@@
 			(layers "F.Cu" "F.Mask" "F.Paste")
 			(roundrect_rratio 0.25)
-			(net 14 "Net-(IC0-OUTPUT_2)")
+			(net 14 "/PHT_DAT_1_R")
 			(pintype "passive")
 		)
@@
 			(layers "F.Cu" "F.Mask" "F.Paste")
 			(roundrect_rratio 0.25)
-			(net 22 "Net-(IC1-OUTPUT_2)")
+			(net 22 "/PHT_DAT_5_R")
 			(pintype "passive")
 		)
@@
 			(layers "F.Cu" "F.Mask" "F.Paste")
 			(roundrect_rratio 0.25)
-			(net 5 "Net-(IC2-OUTPUT_4)")
+			(net 5 "/PHT_DAT_15_R")
 			(pintype "passive")
 		)
@@
 			(layers "F.Cu" "F.Mask" "F.Paste")
 			(roundrect_rratio 0.25)
-			(net 5 "Net-(IC2-OUTPUT_4)")
+			(net 5 "/PHT_DAT_15_R")
 			(pintype "passive")
 		)
@@
 			(layers "F.Cu" "F.Mask" "F.Paste")
 			(roundrect_rratio 0.25)
-			(net 22 "Net-(IC1-OUTPUT_2)")
+			(net 22 "/PHT_DAT_5_R")
 			(pintype "passive")
 		)
@@
 			(layers "F.Cu" "F.Mask" "F.Paste")
 			(roundrect_rratio 0.25)
-			(net 26 "Net-(IC1-OUTPUT_4)")
+			(net 26 "/PHT_DAT_7_R")
 			(pintype "passive")
 		)
@@
 			(layers "F.Cu" "F.Mask" "F.Paste")
 			(roundrect_rratio 0.25)
-			(net 10 "Net-(IC2-OUTPUT_3)")
+			(net 10 "/PHT_DAT_14_R")
 			(pintype "passive")
 		)
@@
 			(layers "F.Cu" "F.Mask" "F.Paste")
 			(roundrect_rratio 0.25)
-			(net 26 "Net-(IC1-OUTPUT_4)")
+			(net 26 "/PHT_DAT_7_R")
 			(pintype "passive")
 		)
@@
 			(layers "F.Cu" "F.Mask" "F.Paste")
 			(roundrect_rratio 0.25)
-			(net 8 "Net-(IC2-OUTPUT_2)")
+			(net 8 "/PHT_DAT_13_R")
 			(pintype "passive")
 		)
@@
 			(layers "F.Cu" "F.Mask" "F.Paste")
 			(roundrect_rratio 0.25)
-			(net 18 "Net-(IC0-OUTPUT_4)")
+			(net 18 "/PHT_DAT_3_R")
 			(pintype "passive")
 		)
@@
 			(layers "F.Cu" "F.Mask" "F.Paste")
 			(roundrect_rratio 0.25)
-			(net 1 "Net-(IC2-OUTPUT_1)")
+			(net 1 "/PHT_DAT_12_R")
 			(pintype "passive")
 		)
@@
 			(layers "F.Cu" "F.Mask" "F.Paste")
 			(roundrect_rratio 0.25)
-			(net 28 "Net-(IC3-OUTPUT_1)")
+			(net 28 "/PHT_DAT_11_R")
 			(pintype "passive")
 		)
